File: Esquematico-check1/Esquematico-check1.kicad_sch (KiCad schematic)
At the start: 20 parts, among them J1 Conn_01x02, J2 Conn_01x02, Q1 BC547, Q2 BC547, Q3 BC547, Q4 BC547, Q5 BC547, Q6 BC557, Q7 BC557, Q8 BC557, U1 TL431D

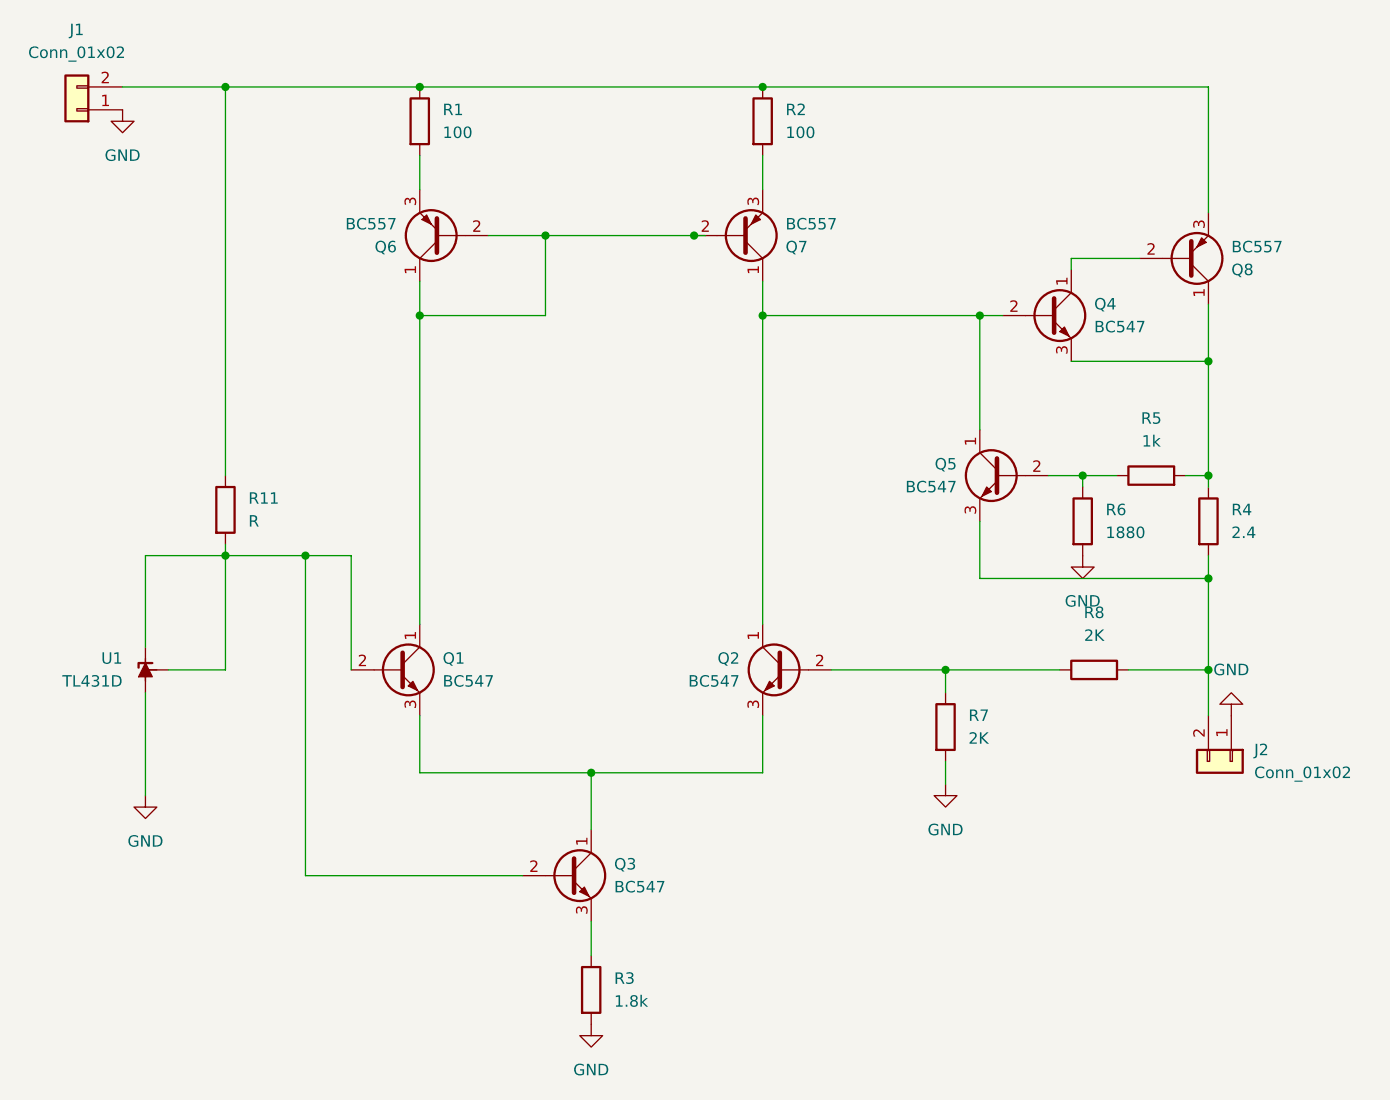
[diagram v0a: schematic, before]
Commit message: esquematico chk1 terminado
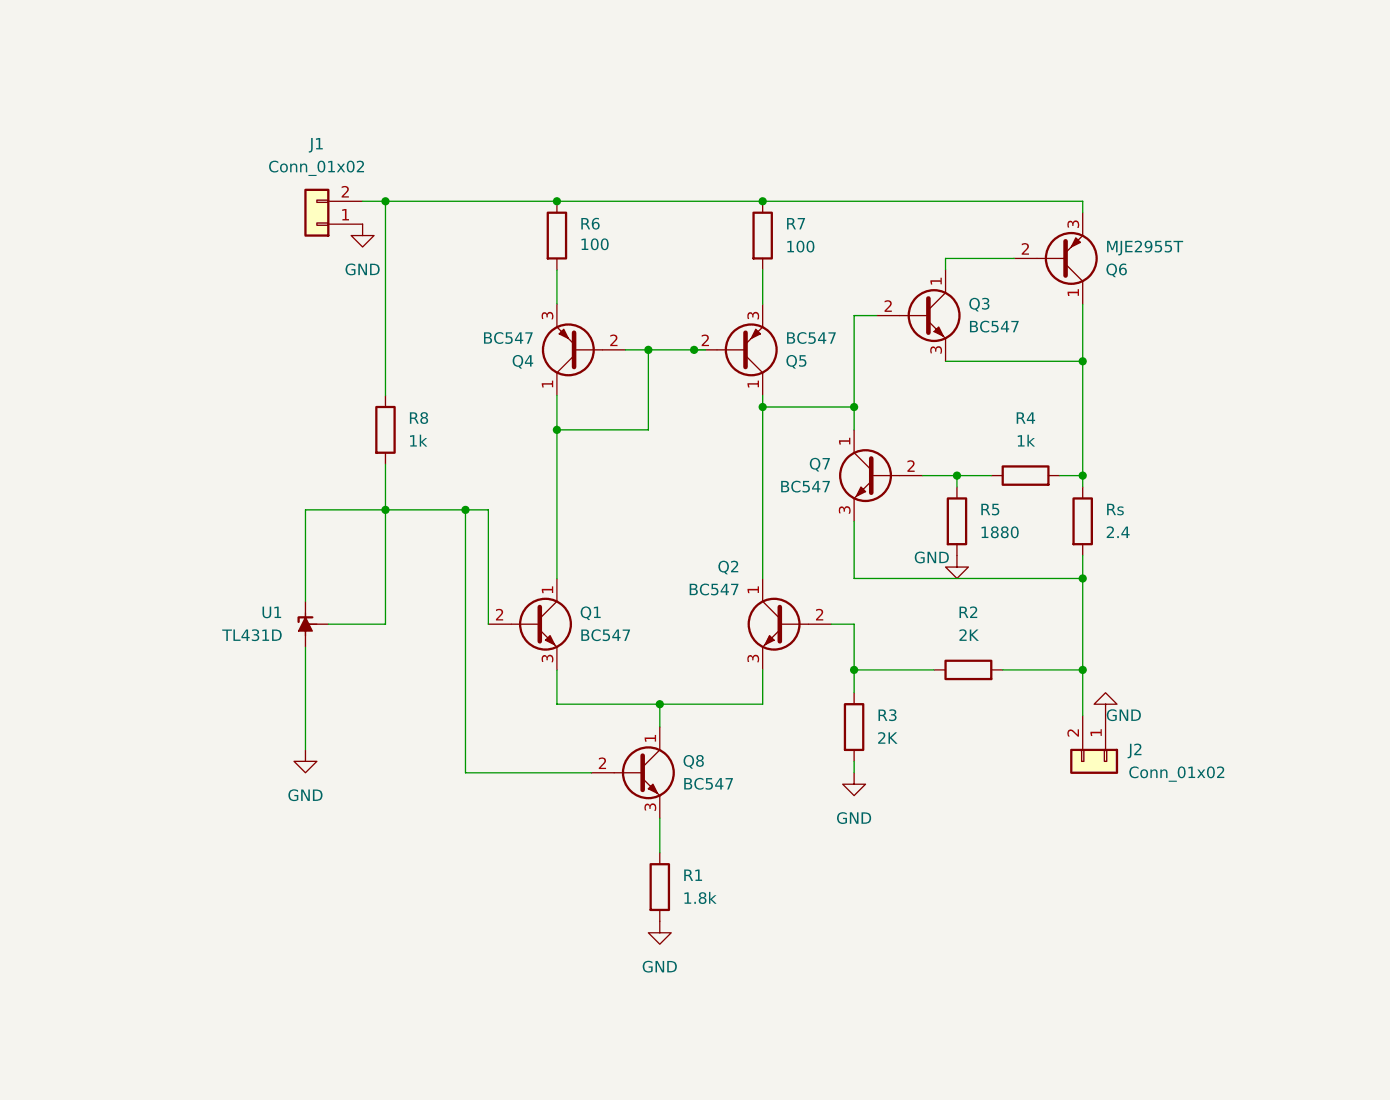
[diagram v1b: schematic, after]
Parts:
- Q4: renamed from Q6; value BC557 -> BC547
- Q5: renamed from Q7; value BC557 -> BC547
- Q6: renamed from Q8; value BC557 -> MJE2955T
- R8: renamed from R11; value R -> 1k
- renumbered Q4 to Q3, Q5 to Q7, Q3 to Q8, R3 to R1, R8 to R2, R7 to R3, R5 to R4, R6 to R5, R1 to R6, R2 to R7, R4 to Rs
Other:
- moved on the sheet: J1, J2, Q1, Q2, Q3, Q4, Q5, Q6, Q7, Q8, R1, R2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
